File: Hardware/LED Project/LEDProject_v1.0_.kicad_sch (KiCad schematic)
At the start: 4 parts, among them J1 Conn_01x02, SW1 SW_Push

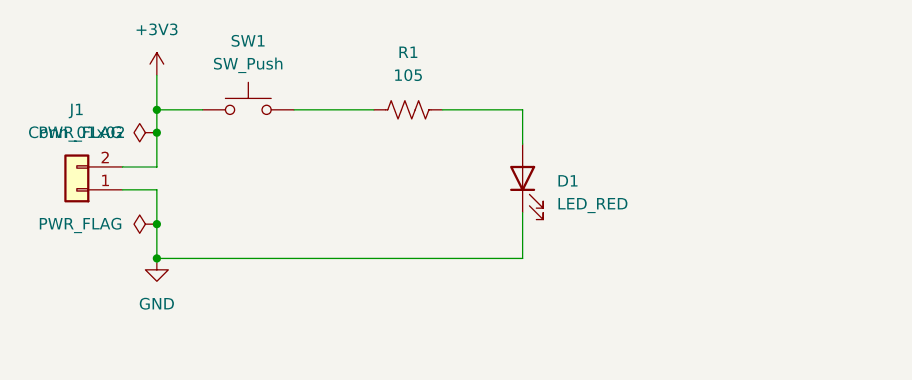
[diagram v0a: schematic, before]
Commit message: LED Project 1 Complete
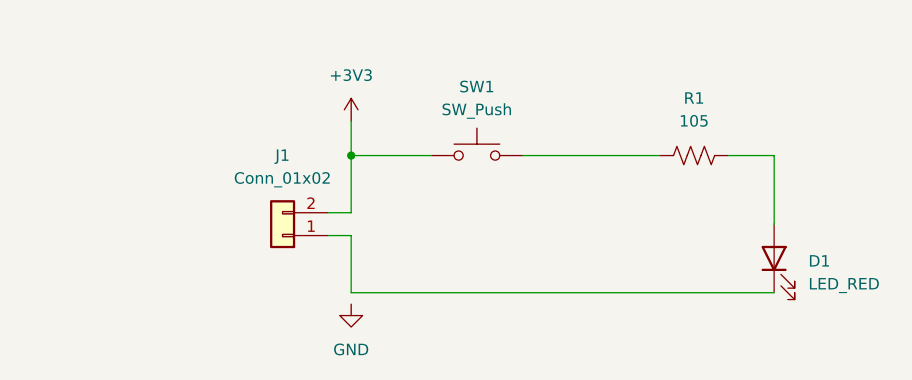
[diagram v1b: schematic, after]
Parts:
- D1: footprint Resistor_SMD:R_0603_1608Metric_Pad0.98x0.95mm_HandSolder -> LED_SMD:LED_0603_1608Metric_Pad1.05x0.95mm_HandSolder
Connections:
- net GND: no longer D1.1 (K), J1.1 (Pin_1)
- new net: D1.1 (K), J1.1 (Pin_1)
